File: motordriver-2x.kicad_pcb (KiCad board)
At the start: 4 copper layers, 215 x 130 mm, 651 parts, among them J1 USB_B_Micro, J2 CONN_RJ45_MAG, J3 CONN_RJ45_MAG, P1 CONN_BUTTON, P11 CONN_JOYSTICK, P13 CONN_SENSOR, P14 CONN_SENSOR, P15 CONN_SENSOR, P16 CONN_SENSOR, P17 CONN_DEBUG_2R, P18 CONN_POWER_41A, P19 CONN_CAN, P2 CONN_BUTTON, P20 CONN_CAN, P21 CONN_AN_OUT, P22 CONN_AN_OUT, P23 CONN_POWER_10A, P24 CONN_CAN, P25 CONN_LCD, P26 CONN_AN_OUT, P27 CONN_AN_OUT, P28 CONN_UEXT, P3 CONN_BUTTON, P37 CONN_ENCODER, P38 CONN_SENSOR, P39 CONN_SENSOR, P4 CONN_BUTTON, P40 CONN_SENSOR, P41 CONN_ENCODER, P42 CONN_SENSOR, P43 CONN_SENSOR, P44 CONN_SENSOR, P45 CONN_MOTOR, P46 CONN_MOTOR, P47 CONN_HALL, P48 CONN_HALL, P49 CONN_BRKRES, P5 CONN_BUTTON, P6 CONN_BUTTON, P7 CONN_BUTTON, P8 CONN_BUTTON, P9 CONN_JOYSTICK, Q1 Q_NMOS_2X_60V_63A, Q2 Q_NMOS_2X_60V_63A, Q3 Q_NMOS_2X_60V_63A, Q4 Q_NMOS_2X_60V_63A, Q5 Q_NMOS_2X_60V_63A, Q6 Q_NMOS_2X_60V_63A, Q7 Q_PNP_BC856, Q8 Q_NMOS_BUK9875, U1 IC_MIC2026, U10 IC_MCP4461, U11 IC_MCP2517FD-xJHA, U12 IC_STM32F429ZET6, U13 IC_MCP23S17, U14 IC_TPS54360DDA, U15 IC_TJA1044GT3, U16 IC_TLV2474, U17 IC_M24C16, U18 IC_USBLC6-2, U19 IC_TPS62147RGXR, U2 IC_MAX6818, U20 IC_TLV75533, U21 IC_LP55231, U22 IC_TLV75533, U23 IC_MAX14890, U24 IC_MAX14890, U25 IC_MIC2026, U26 IC_TLV2474, U27 IC_USBLC6-2, U28 IC_USBLC6-2, U29 IC_MCP4461, U3 IC_TLV2474, U30 IC_LAN9252, U31 IC_DRV8302, U32 IC_DRV8302, U33 IC_TLV2474, U34 IC_M24C16, U35 IC_TLV2474, U36 IC_TLV75533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

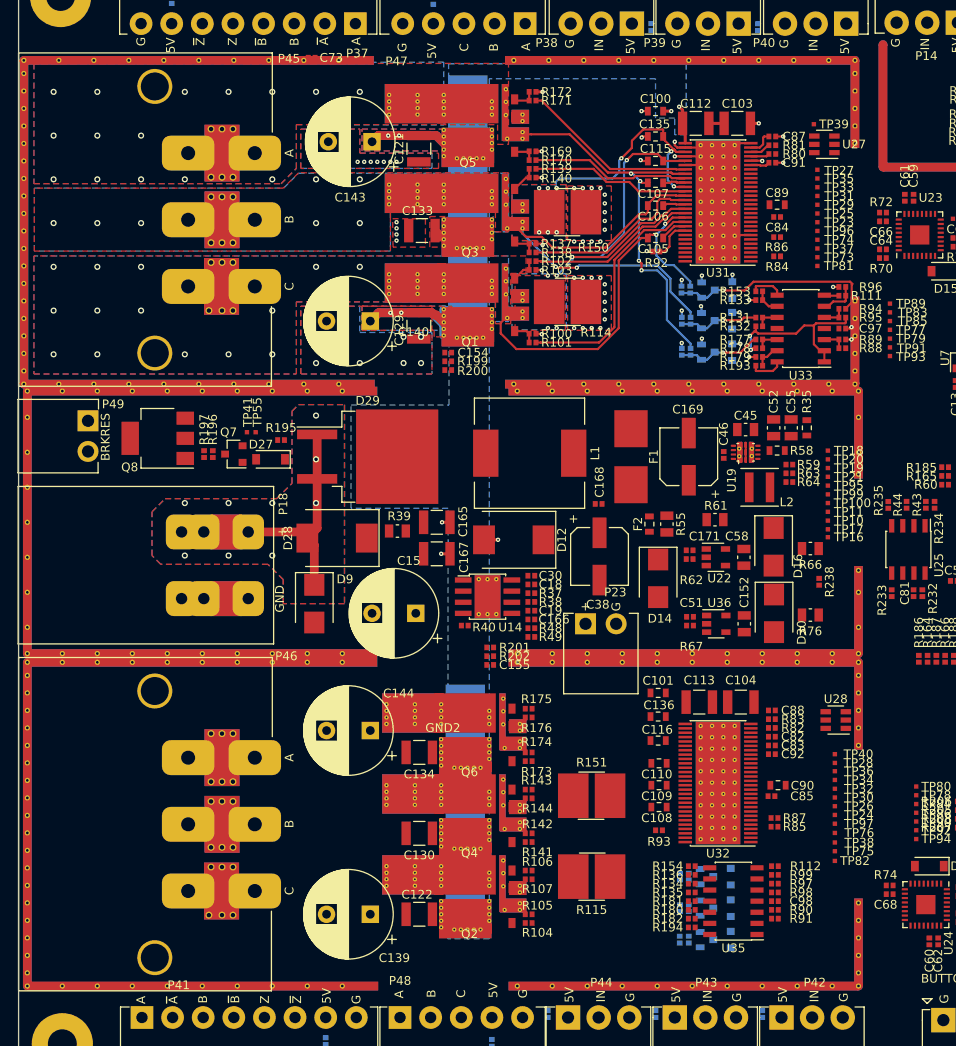
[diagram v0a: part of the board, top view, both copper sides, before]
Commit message: routing power supply
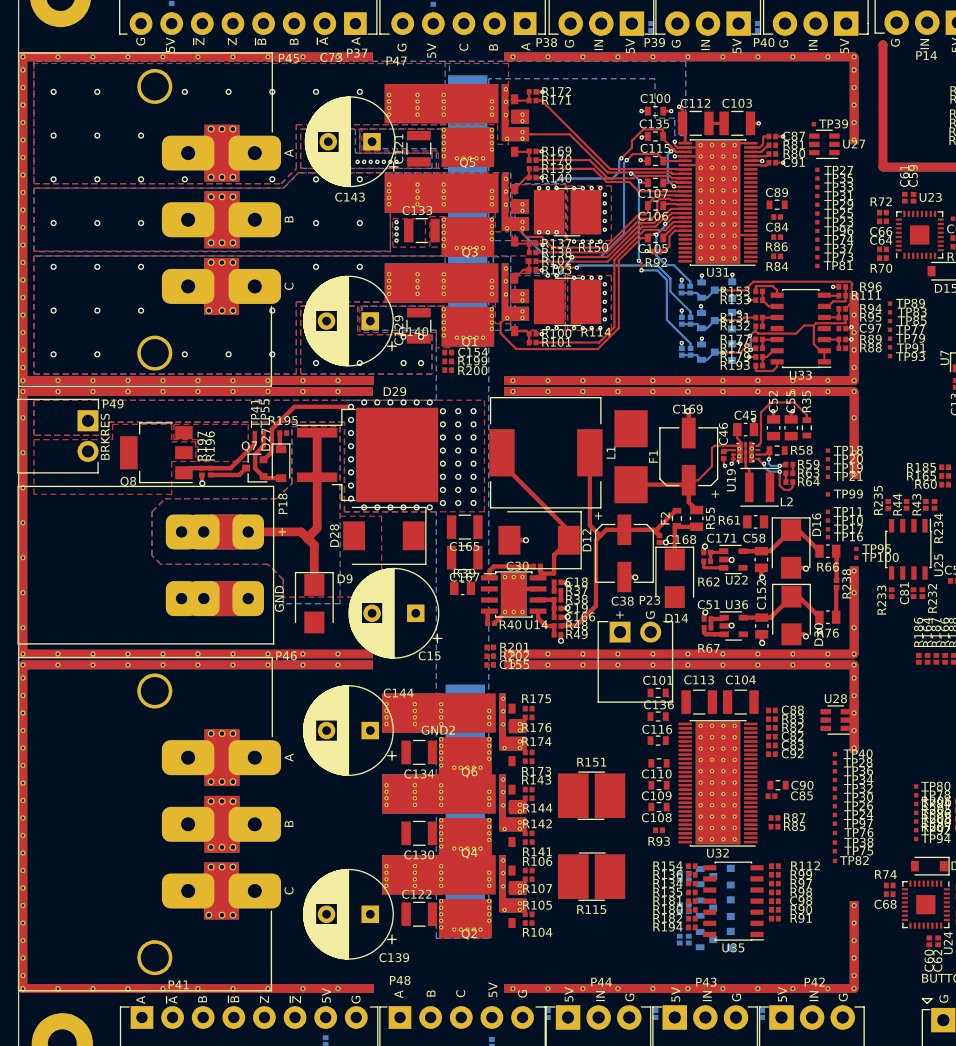
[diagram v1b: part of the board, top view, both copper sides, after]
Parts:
- moved R39 9.92 mm to (96.8, 96.8)
- moved C168 8.03 mm to (119.2, 91.1), turned to 270 degrees
- moved TP95 7.95 mm to (141.8, 92.2)
- moved TP100 7.04 mm to (141.8, 93.2)
- moved D28 5.36 mm to (87.8, 90.8)
- moved R61 4.66 mm to (130.2, 89.2)
- moved P23 4.06 mm to (114.8, 101.8)
- moved R55 3.46 mm to (123.5, 88.8)
- moved C165 3.25 mm to (97.0, 89.8), turned to 180 degrees
- moved C167 3.23 mm to (97.0, 93.2), turned to 180 degrees
- moved F2 3.22 mm to (121.2, 88.8)
- moved C166 3.01 mm to (107.6, 100.0)
- moved C18 3.01 mm to (107.6, 96.0)
- moved C19 3.01 mm to (107.6, 99.0)
- moved R37 3.01 mm to (107.6, 97.0)
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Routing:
- net VMOT: track 127.7 -> 20.4 mm, vias 6 -> 46
- net GND: track 36.4 -> 72.2 mm, vias 76 -> 97
- net Net-(C168-Pad1): track 0.00 -> 34.1 mm
- net Net-(C169-Pad1): track 0.00 -> 22.6 mm
- net Net-(C30-Pad1): track 0.00 -> 20.6 mm
- net Net-(R35-Pad2): track 0.00 -> 10.9 mm
- net Net-(C58-Pad1): track 0.00 -> 10.7 mm
- net Net-(Q8-Pad1): track 0.00 -> 10.7 mm
- net Net-(C152-Pad1): track 0.00 -> 10.7 mm
- net Net-(D27-Pad2): track 0.00 -> 7.85 mm
- net Net-(D14-Pad1): track 0.00 -> 6.21 mm
- net Net-(R58-Pad2): track 0.00 -> 6.05 mm, vias 0 -> 2
- net Net-(C30-Pad2): track 0.00 -> 6.05 mm
- net USB_5V: track 0.00 -> 5.15 mm
- net Net-(Q7-Pad3): track 0.00 -> 4.38 mm
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- added copper zone on F.Cu, net Net-(P49-Pad2)
